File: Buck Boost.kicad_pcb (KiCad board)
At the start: 2 copper layers, 105.7 x 75.9 mm, 41 parts, among them J1 DC IN, J2 DC 5V, J3 OUT, J4 TRACO DC IN, K1 SW_SPDT, K2 Jumper_2_Bridged, T2 IRF4905S, T3 IRF4905S, U1 HCPL-3120, U2 arduino, U3 HCPL-3120, U4 ER_OLEDM0.91_1x-I2C, U5 TMA-1512S

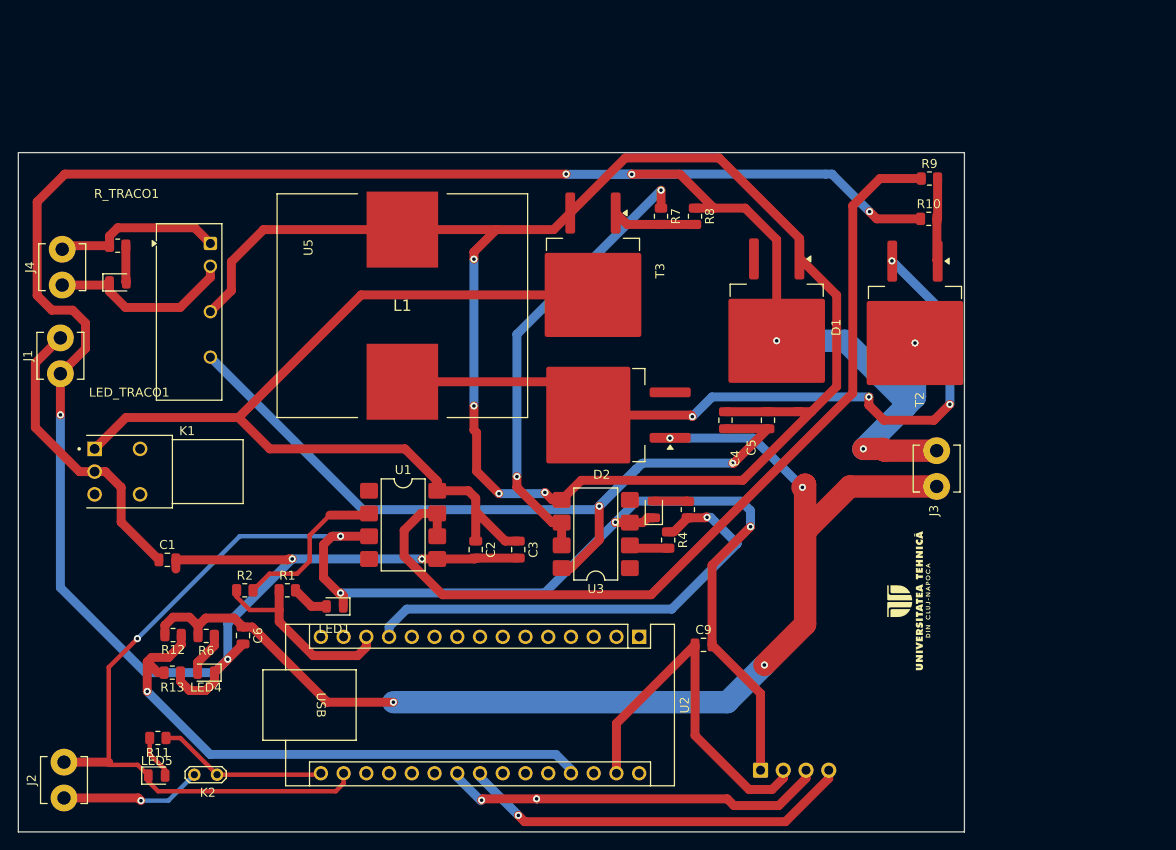
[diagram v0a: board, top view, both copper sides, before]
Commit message: final 1
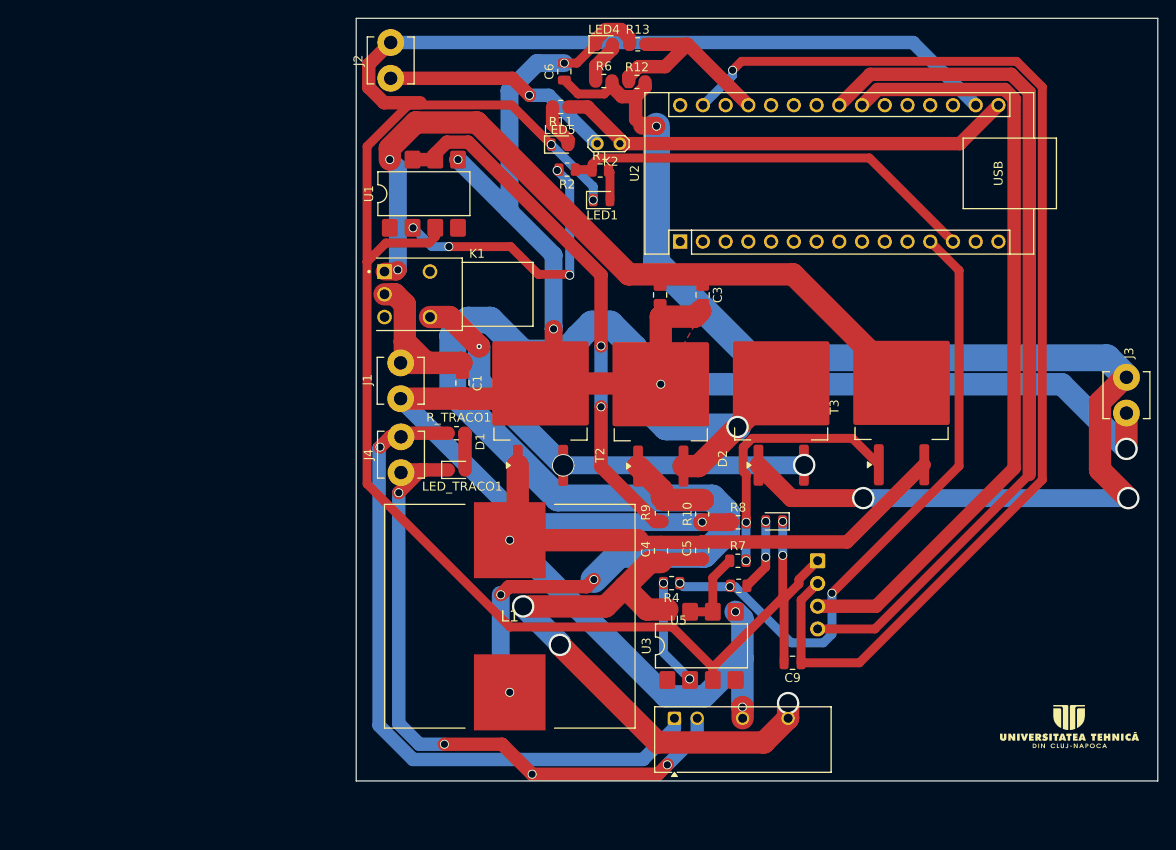
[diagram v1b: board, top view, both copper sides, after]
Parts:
- moved J2 88.3 mm to (155.9, 41.8)
- moved R13 87.4 mm to (183.5, 38.0), turned to 0 degrees
- moved LED5 83.6 mm to (174.8, 49.2)
- moved R11 83.6 mm to (174.9, 45.0)
- moved K2 83.6 mm to (181.5, 49.1)
- moved LED4 83.1 mm to (179.7, 38.0), turned to 0 degrees
- moved R12 80.7 mm to (183.4, 42.2), turned to 0 degrees
- moved R6 76.3 mm to (179.7, 42.1), turned to 0 degrees
- moved U5 74.2 mm to (187.6, 113.3), turned to 90 degrees
- moved C6 72.5 mm to (175.3, 41.0), turned to 90 degrees
- moved R2 59.2 mm to (175.6, 52.0), turned to 180 degrees
- moved R1 58.5 mm to (179.3, 52.1)
- moved LED1 54.3 mm to (179.5, 55.4), turned to 0 degrees
- moved R9 47.9 mm to (186.2, 90.4), turned to 90 degrees
- moved U2 44.4 mm to (188.2, 60.0), turned to 90 degrees
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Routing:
- net Net-(D1-A): track 314.2 -> 205.0 mm, vias 10 -> 6
- net Net-(U2-3V3): track 41.9 -> 130.4 mm, vias 0 -> 1
- net Net-(D1-K): track 181.5 -> 106.0 mm, vias 4 -> 3
- net Net-(J2-Pin_1): track 178.7 -> 242.0 mm, vias 5 -> 4
- net Net-(J4-Pin_2): track 18.9 -> 76.5 mm, vias 0 -> 1
- net Net-(D2-A): track 86.0 -> 142.1 mm
- net Net-(J4-Pin_1): track 21.2 -> 74.5 mm, vias 0 -> 4
- net Net-(U2-A4): track 44.4 -> 97.0 mm, vias 1 -> 0
- net (no net): track 0.00 -> 51.0 mm, vias 0 -> 3
- net Net-(U2-A5): track 43.0 -> 87.8 mm, vias 2 -> 0
- net Net-(R7-Pad1): track 51.0 -> 9.02 mm, vias 2 -> 0
- net Net-(R9-Pad1): track 101.0 -> 59.2 mm, vias 0 -> 2
- net Net-(U2-A0): track 62.7 -> 22.9 mm, vias 1 -> 0
- net Net-(K2-A): track 19.1 -> 52.0 mm
- net Net-(U3-VCC): track 93.0 -> 66.7 mm, vias 2 -> 3
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- added copper zone on F.Cu, net Net-(D1-A)
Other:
- board size 105.7 x 75.9 mm -> 89.5 x 85.2 mm
